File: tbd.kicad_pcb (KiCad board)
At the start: 2 copper layers, 22.6 x 12 mm, 8 parts, among them J1 USBPCB, P1 CONN_02X04, U1 MKL27ZxxxVFM4

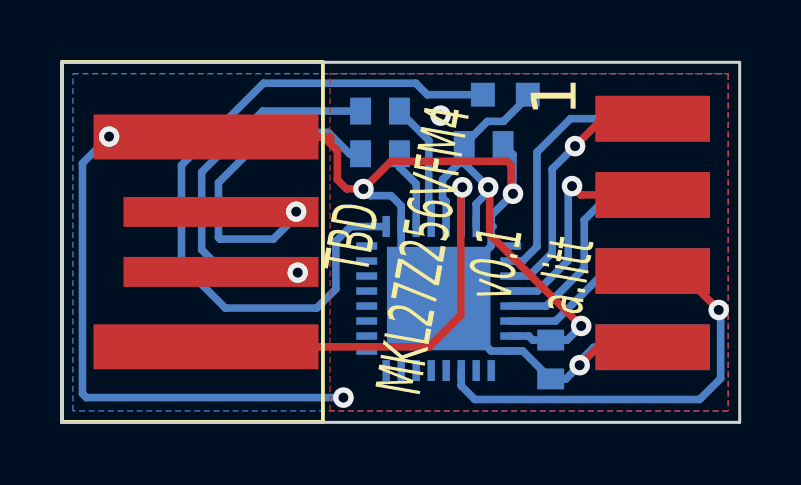
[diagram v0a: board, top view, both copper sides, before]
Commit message: Update design to v0.2
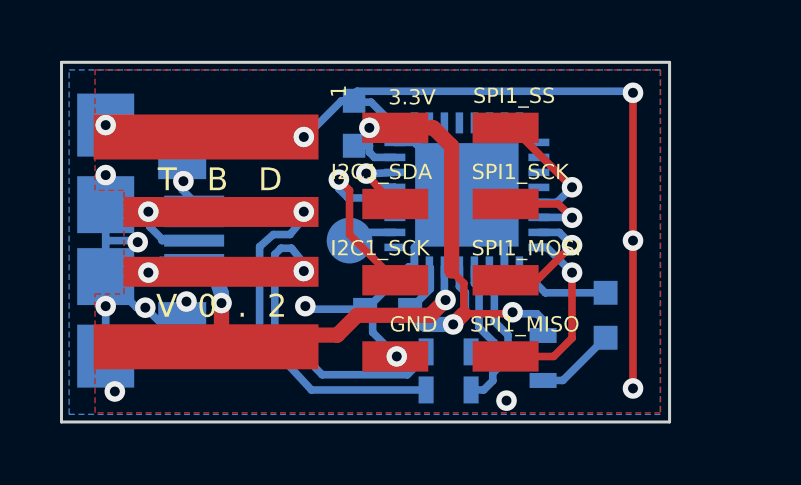
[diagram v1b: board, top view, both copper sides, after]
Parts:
- added J2: USB-MICROB-5PIN, tbd:SparkFun-USB-MICROB, B.Cu at (107.9, 94.8)
- added R3: 33R, tbd:R_0603, B.Cu at (119.3, 98.6)
- added SWD_CLK: SWD_CLK, Measurement_Points:Measurement_Point_Round-SMD-Pad_Small, B.Cu at (116.0, 94.8)
- C1, C2: footprint tbd:SparkFun-0402-CAP -> tbd:C_0603
- LED1: footprint tbd:SparkFun-LED-0402 -> tbd:LED-0603
- P1: footprint tbd:hdr-boardedge-4x2 -> tbd:HEADER_2x4_SMT_RA
- R1: value 33R -> 100R; footprint tbd:SparkFun-0402-RES -> tbd:R_0603
- R2: footprint tbd:SparkFun-0402-RES -> tbd:R_0603
- moved C2 10.2 mm to (116.2, 90.9), turned to 90 degrees
- moved R2 9.57 mm to (119.3, 99.8)
- moved P1 9.27 mm to (117.6, 91.1), turned to 90 degrees
- moved R1 8.71 mm to (122.5, 98.8), turned to 270 degrees
- moved LED1 8.08 mm to (124.6, 97.3), turned to 90 degrees
- moved C1 6.35 mm to (117.3, 97.1), turned to 180 degrees
- moved U1 3.58 mm to (119.9, 93.3), turned to 90 degrees
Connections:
- LED1 pad A: +3.3V -> Net-(LED1-PadA)
- P1 pad 1: LPUART0_RX -> +3.3V
- P1 pad 2: SWD_CLK -> SPI1_SS
- P1 pad 3: LPUART0_TX -> I2C1_SDA
- P1 pad 4: SWD_DIO -> SPI1_SCK
- P1 pad 5: /RESET -> I2C1_SCL
- P1 pad 6: /NMI -> SPI1_MOSI
- P1 pad 8: VSS -> SPI1_MISO
- R1 pad 1: Net-(J1-PadDP) -> +3.3V
- R1 pad 2: Net-(R1-Pad2) -> Net-(LED1-PadA)
- R2 pad 1: Net-(J1-PadDN) -> Net-(J1-PadDP)
- U1 pad 10: SWD_CLK -> Net-(TP1-Pad1)
- U1 pad 11: LPUART0_RX -> (no net)
- U1 pad 12: LPUART0_TX -> (no net)
- U1 pad 13: SWD_DIO -> I2C1_SCL
- U1 pad 14: /NMI -> I2C1_SDA
- U1 pad 19: /RESET -> (no net)
- U1 pad 29: (no net) -> SPI1_SS
- U1 pad 3: Net-(R1-Pad2) -> Net-(R2-Pad2)
- U1 pad 30: (no net) -> SPI1_SCK
- U1 pad 31: (no net) -> SPI1_MOSI
- U1 pad 32: (no net) -> SPI1_MISO
- U1 pad 4: Net-(R2-Pad2) -> Net-(R3-Pad2)
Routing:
- net Net-(LED1-PadC): track 24.1 -> 3.23 mm
- net /RESET: track 16.9 -> 0.00 mm, vias 1 -> 0
- net SWD_DIO: track 11.6 -> 0.00 mm
- net LPUART0_RX: track 10.2 -> 0.00 mm, vias 1 -> 0
- net SWD_CLK: track 8.55 -> 0.00 mm
- net LPUART0_TX: track 7.68 -> 0.00 mm, vias 1 -> 0
- net I2C1_SCL: track 0.00 -> 6.63 mm, vias 0 -> 1
- net SPI1_MISO: track 0.00 -> 6.38 mm, vias 0 -> 1
- net Net-(J1-PadDP): track 17.9 -> 23.7 mm, vias 1 -> 2
- net /NMI: track 5.43 -> 0.00 mm
- net SPI1_SS: track 0.00 -> 4.35 mm, vias 0 -> 1
- net SPI1_MOSI: track 0.00 -> 3.98 mm, vias 0 -> 1
- net Net-(R3-Pad2): track 0.00 -> 3.95 mm
- net VSS: track 65.4 -> 69.2 mm, vias 5 -> 14
- net SPI1_SCK: track 0.00 -> 3.51 mm, vias 0 -> 1
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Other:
- board size 22.6 x 12 mm -> 20.3 x 12 mm
- net class pwr added: clearance 0.127, trace_width 0.508, via_dia 0.6858, via_drill 0.3302
- board text added: "3.3V"
- board text added: "GND"
- board text added: "I2C1_SCK"
- board text added: "I2C1_SDA"
- board text added: "SPI1_MISO"
- board text added: "SPI1_MOSI"
- board text added: "SPI1_SCK"
- board text added: "SPI1_SS"
- board text added: "T B D"
- board text added: "V 0 . 2"
- board text removed: "1"
- board text removed: "TBD MKL27Z256VFM4 v0.1 a.litt"
